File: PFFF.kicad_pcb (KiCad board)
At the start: 2 copper layers, 25 x 22.9 mm, 15 parts, among them J1 Conn_01x02, J2 Conn_01x02, J3 Conn_01x03, J4 Conn_01x03, U1 TPS61099YFFT

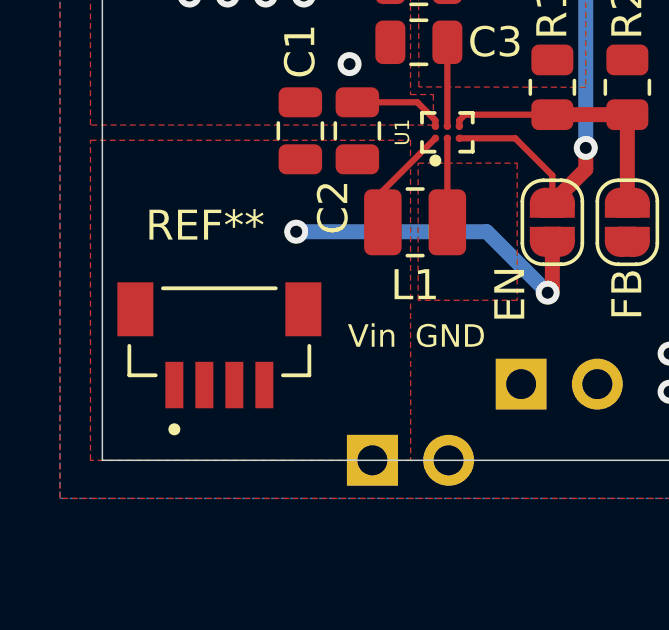
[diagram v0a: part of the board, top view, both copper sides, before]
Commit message: Revert "fake add component"
This reverts commit 96a2ccfc30ab2f58efbd566c060a8c6ea30395aa.
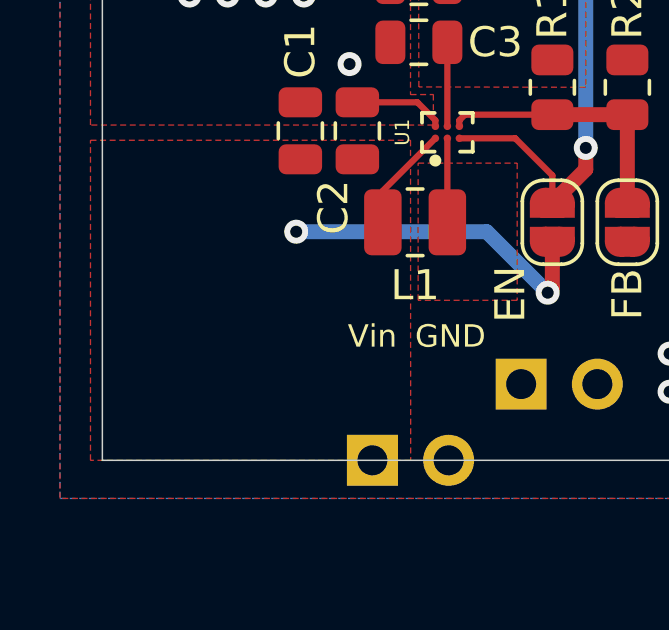
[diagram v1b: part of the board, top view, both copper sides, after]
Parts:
- removed REF**: JST_BM04B-SRSS-TB_LF__SN_, Snapeda:BM04B-SRSS-TB_LF__SN__JST_BM04B-SRSS-TB_LF__SN_

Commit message: fake add component
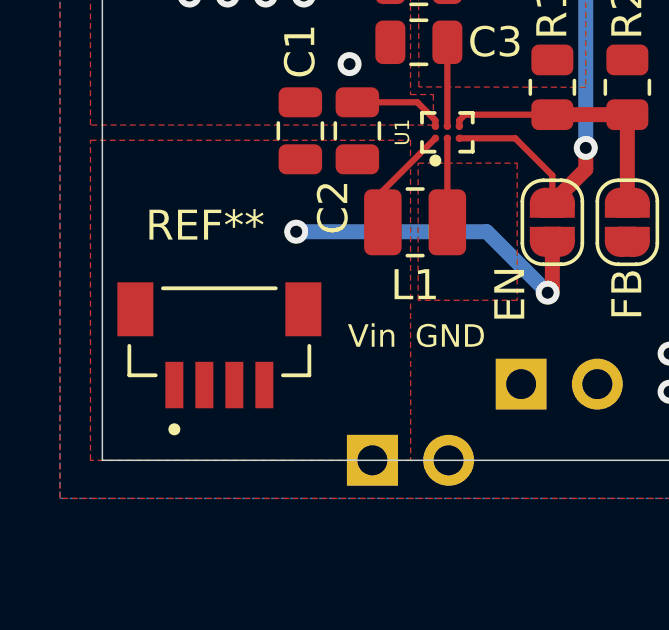
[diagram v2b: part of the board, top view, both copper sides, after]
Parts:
- added REF**: JST_BM04B-SRSS-TB_LF__SN_, Snapeda:BM04B-SRSS-TB_LF__SN__JST_BM04B-SRSS-TB_LF__SN_, F.Cu at (137.9, 101.9)
